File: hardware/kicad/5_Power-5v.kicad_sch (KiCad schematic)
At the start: 20 parts, among them Q32 DMN4800LSSL-13, U103 220uF, U47 LM74700QDBVRQ1, U49 8mΩ

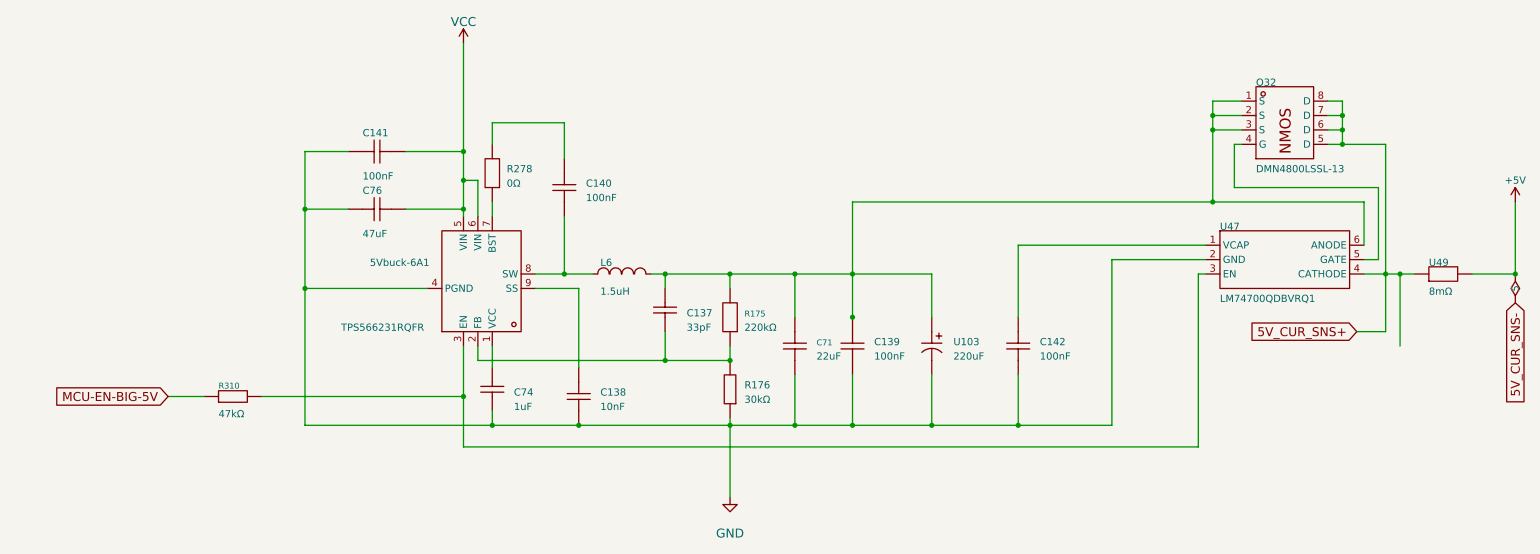
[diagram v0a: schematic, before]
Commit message: sub modules
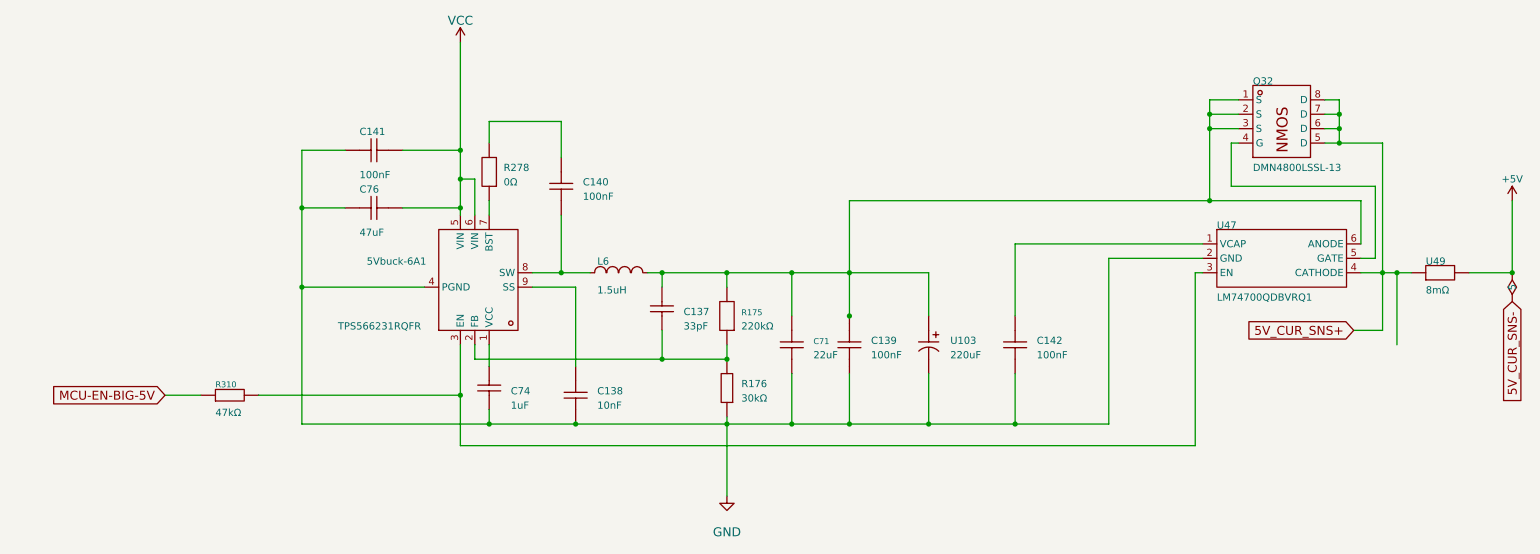
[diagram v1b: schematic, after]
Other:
- moved on the sheet: 5, 5Vbuck-6A1, C137, C138, C139, C140, C141, C142, C71, C74, C76, L6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
